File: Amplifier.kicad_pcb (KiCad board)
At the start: 2 copper layers, 68 x 50 mm, 28 parts, among them J1 Input, J2 Power, J3 Transformer, J4 Neon bulb, U1 6N2P, U2 6P14P

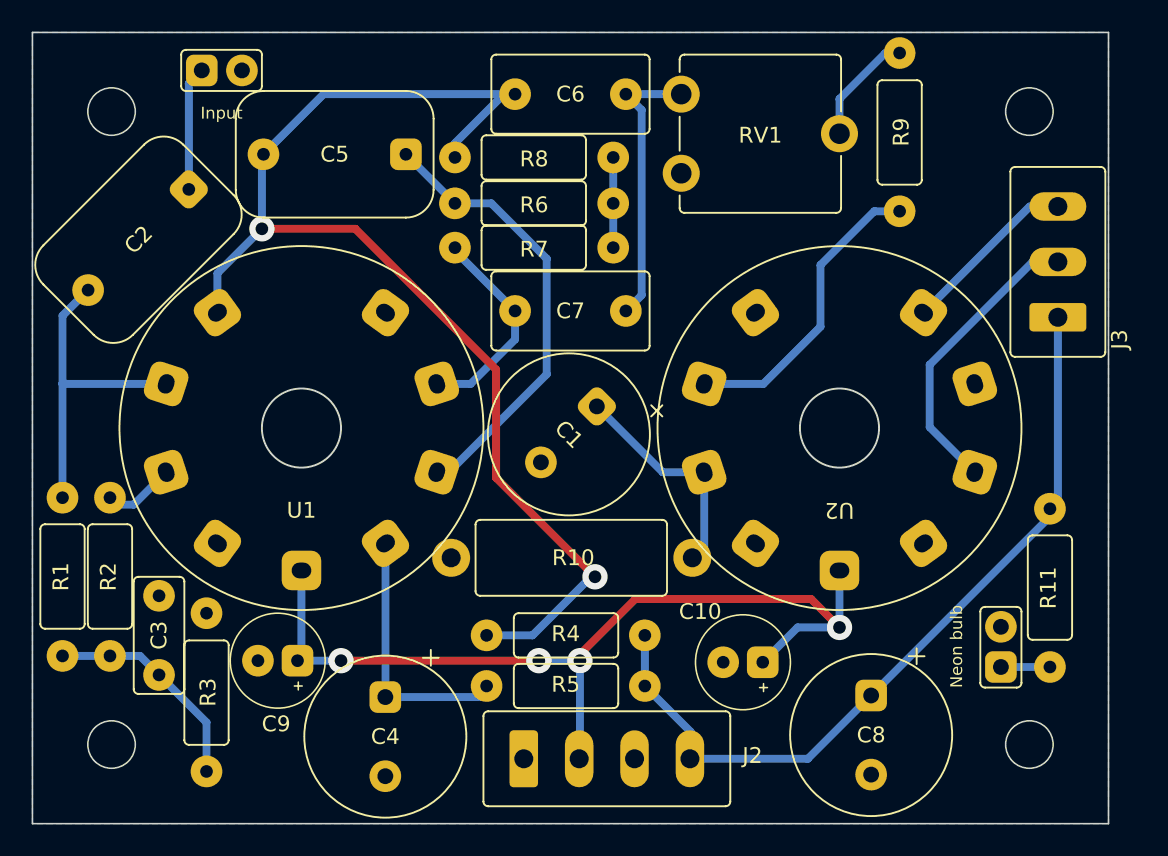
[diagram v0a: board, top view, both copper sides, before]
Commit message: New Amplifier PCB almost ready
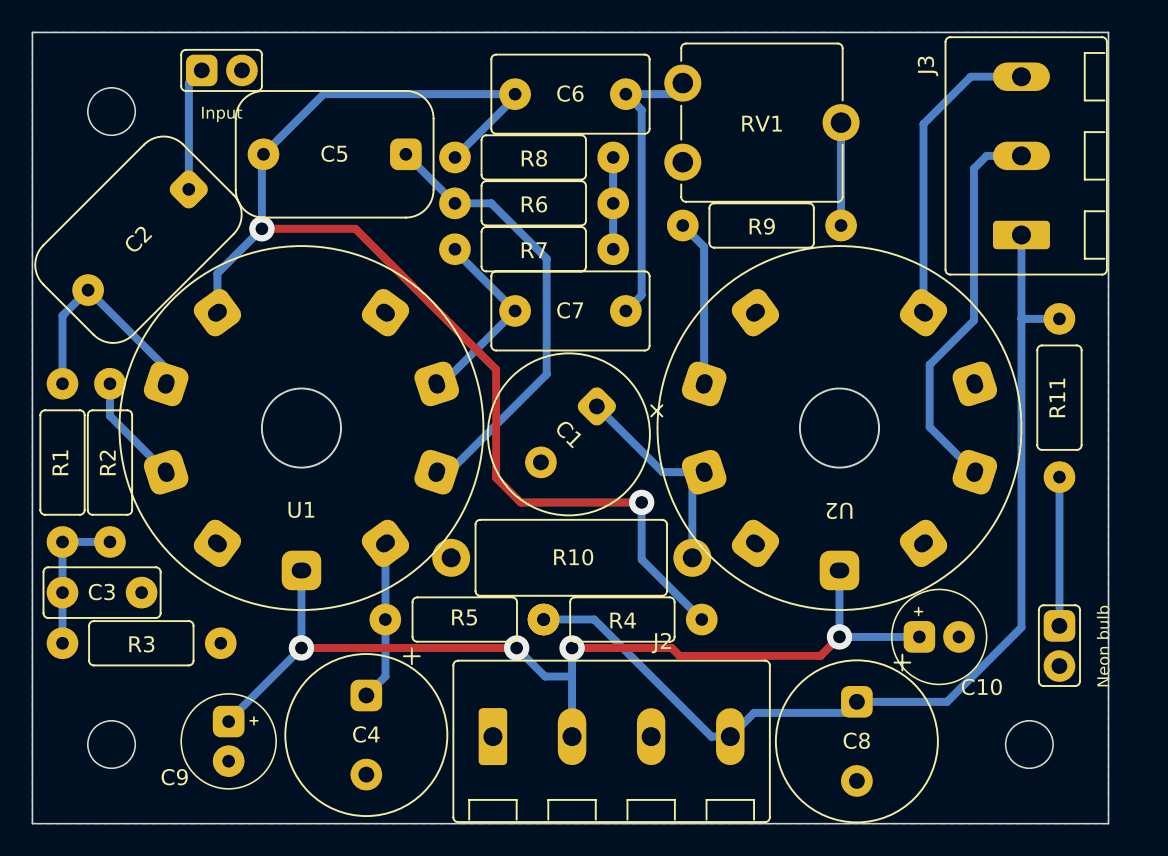
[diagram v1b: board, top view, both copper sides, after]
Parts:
- J2: footprint spdf1626_lib:MCV_1,5_4-G-3.5_1x04_P3.50mm_Vertical -> spdf1626_lib:MCV_1,5_4-G-5.0_1x04_P5.0mm_Vertical
- J3: footprint spdf1626_lib:MCV_1,5_4-G-3.5_1x03_P3.50mm_Vertical -> spdf1626_lib:MCV_1,5_4-G-5.0_1x03_P5.0mm_Vertical
- moved C10 12.5 mm to (114.3, 85.2), turned to 0 degrees
- moved R11 12.0 mm to (121.9, 70.1)
- moved R9 10.5 mm to (103.1, 59.2), turned to 180 degrees
- moved C3 8.02 mm to (58.9, 82.4), turned to 0 degrees
- moved R5 7.66 mm to (84.3, 84.1)
- moved R1 7.20 mm to (58.9, 74.2)
- moved R2 7.20 mm to (61.9, 74.2)
- moved J3 7.08 mm to (119.5, 54.8)
- moved C9 5.97 mm to (69.4, 91.8), turned to -90 degrees
- moved R3 5.14 mm to (63.9, 85.6), turned to 180 degrees
- moved J4 4.52 mm to (121.9, 84.5), turned to 0 degrees
- moved R4 3.74 mm to (94.3, 84.1), turned to 180 degrees
- moved J2 1.43 mm to (93.6, 91.5)
- moved C4 1.20 mm to (78.1, 91.4)
- moved C8 0.98 mm to (109.1, 91.8)
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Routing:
- net 240V: track 50.9 -> 63.6 mm
- net Net-(R9-Pad2): track 19.2 -> 10.6 mm
- net Net-(U2-Pad9): track 11.3 -> 19.3 mm
- net Net-(C4-Pad1): track 16.6 -> 10.1 mm
- net Net-(J4-Pad1): track 3.10 -> 9.40 mm
- net Net-(U2-Pad7): track 18.8 -> 24.9 mm
- net Net-(C2-Pad2): track 20.3 -> 14.6 mm
- net Net-(C3-Pad1): track 13.9 -> 9.40 mm
- net +6V: track 58.2 -> 61.8 mm
- net Net-(R2-Pad2): track 4.58 -> 7.06 mm
- net Net-(C5-Pad2): track 77.2 -> 78.4 mm
- net Net-(C7-Pad1): track 13.5 -> 12.3 mm
- net Net-(R9-Pad1): track 7.20 -> 6.50 mm
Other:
- outline, holes or cut-outs redrawn
